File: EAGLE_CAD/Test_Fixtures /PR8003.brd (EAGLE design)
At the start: 116 x 100 mm, 43 parts, among them J1 M3_SCREW_POST

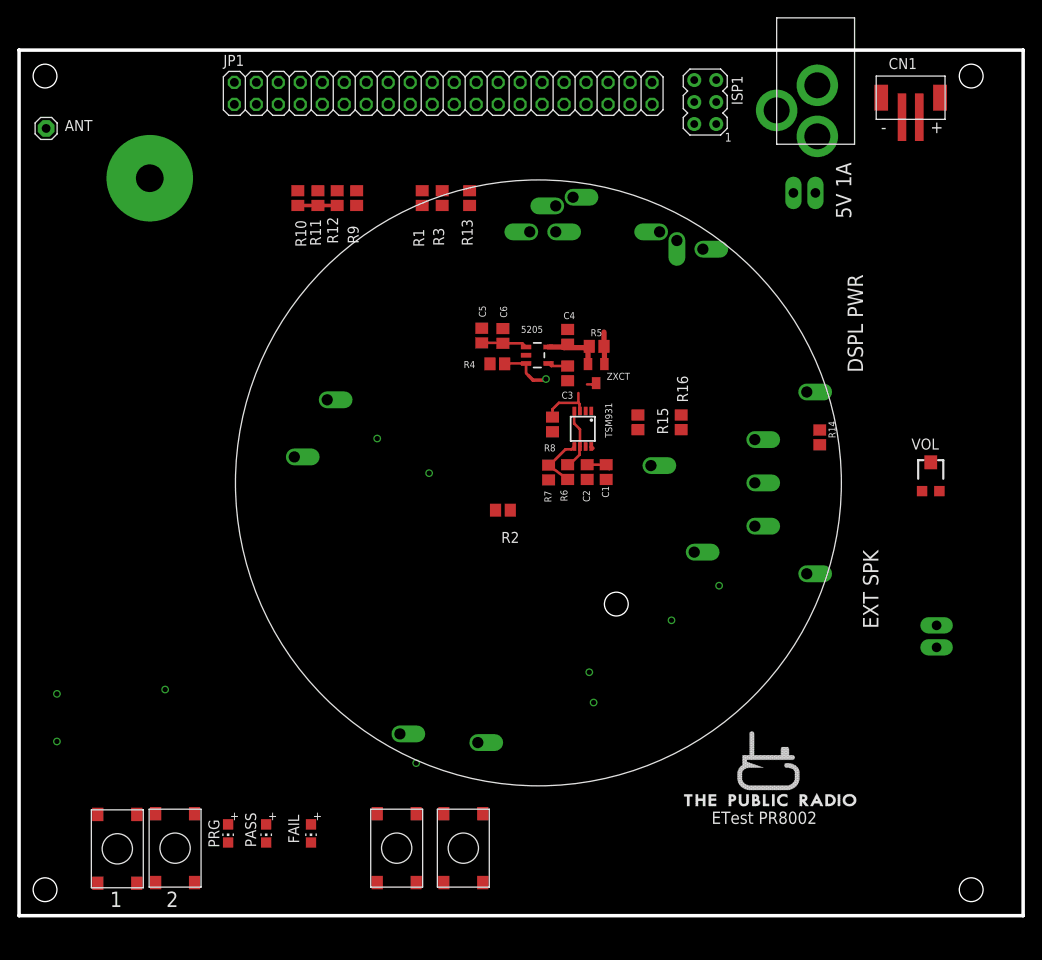
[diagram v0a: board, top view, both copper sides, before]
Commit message: Bumped to PR8003
New layout
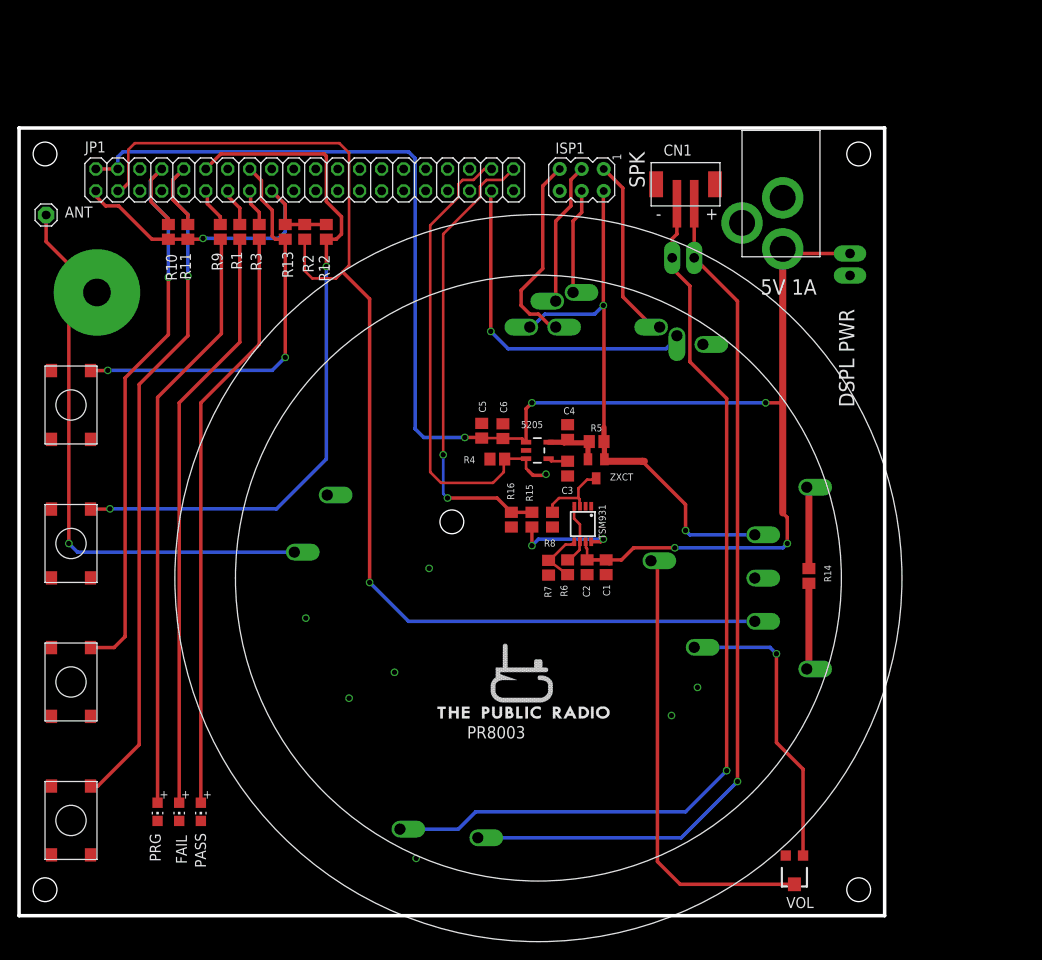
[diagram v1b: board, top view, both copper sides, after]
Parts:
- moved JP2 53.0 mm to (78.0, 76.0), turned to 180 degrees
- moved U$24 51.6 mm to (6.00, 59.0)
- moved VOL 48.4 mm to (89.6, 5.12), turned to 180 degrees
- moved U$23 45.4 mm to (6.00, 11.0)
- moved U$20 42.2 mm to (6.00, 27.0)
- moved R2 39.5 mm to (33.0, 79.0), turned to 270 degrees
- moved U$22 37.2 mm to (6.00, 43.0)
- moved U$1 30.2 mm to (58.1, 28.4)
- moved CN1 27.9 mm to (77.0, 85.0)
- moved R16 22.6 mm to (56.9, 45.8)
- moved R13 21.7 mm to (30.8, 79.0), turned to 270 degrees
- moved R3 21.5 mm to (27.8, 79.0), turned to 270 degrees
- moved R1 21.4 mm to (25.5, 79.0), turned to 270 degrees
- moved JP1 18.9 mm to (33.0, 85.0)
- moved ISP1 16.9 mm to (65.0, 85.0), turned to 270 degrees
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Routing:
- net +5V: track 8.02 -> 188.4 mm, vias 0 -> 5
- net DEV_PRES: track 0.00 -> 138.0 mm, vias 0 -> 1
- net SPK_OUT+: track 0.00 -> 108.9 mm, vias 0 -> 1
- net SPK_OUT-: track 0.00 -> 103.7 mm, vias 0 -> 1
- net TAC2: track 0.00 -> 85.4 mm, vias 0 -> 1
- net TAC3: track 0.00 -> 81.5 mm, vias 0 -> 2
- net TAC1: track 0.00 -> 69.8 mm, vias 0 -> 1
- net ANT: track 0.00 -> 68.3 mm, vias 0 -> 1
- net N$2: track 0.00 -> 68.2 mm
- net N$3: track 0.00 -> 68.0 mm
- net N$4: track 0.00 -> 67.9 mm
- net 3.3V: track 4.76 -> 64.6 mm, vias 0 -> 2
- net COMPARATOR: track 0.00 -> 53.1 mm, vias 0 -> 2
- net A_OUT: track 0.00 -> 52.0 mm
- net REG_ENABLE: track 6.30 -> 56.6 mm
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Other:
- board size 116 x 100 mm -> 100 x 91 mm
- board text added: "PR8003"
- board text added: "SPK"
- board text removed: "1"
- board text removed: "2"
- board text removed: "ETest PR8002"
- board text removed: "EXT SPK"
